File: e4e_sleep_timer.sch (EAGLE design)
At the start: 22 parts, among them P1 XT60, P2 10129378-906001BLF, P3 XT30PW-F, Q1 PJA3416AE_R1_00001, U1 NUCLEO-G071RB, U2 1224-5-150W

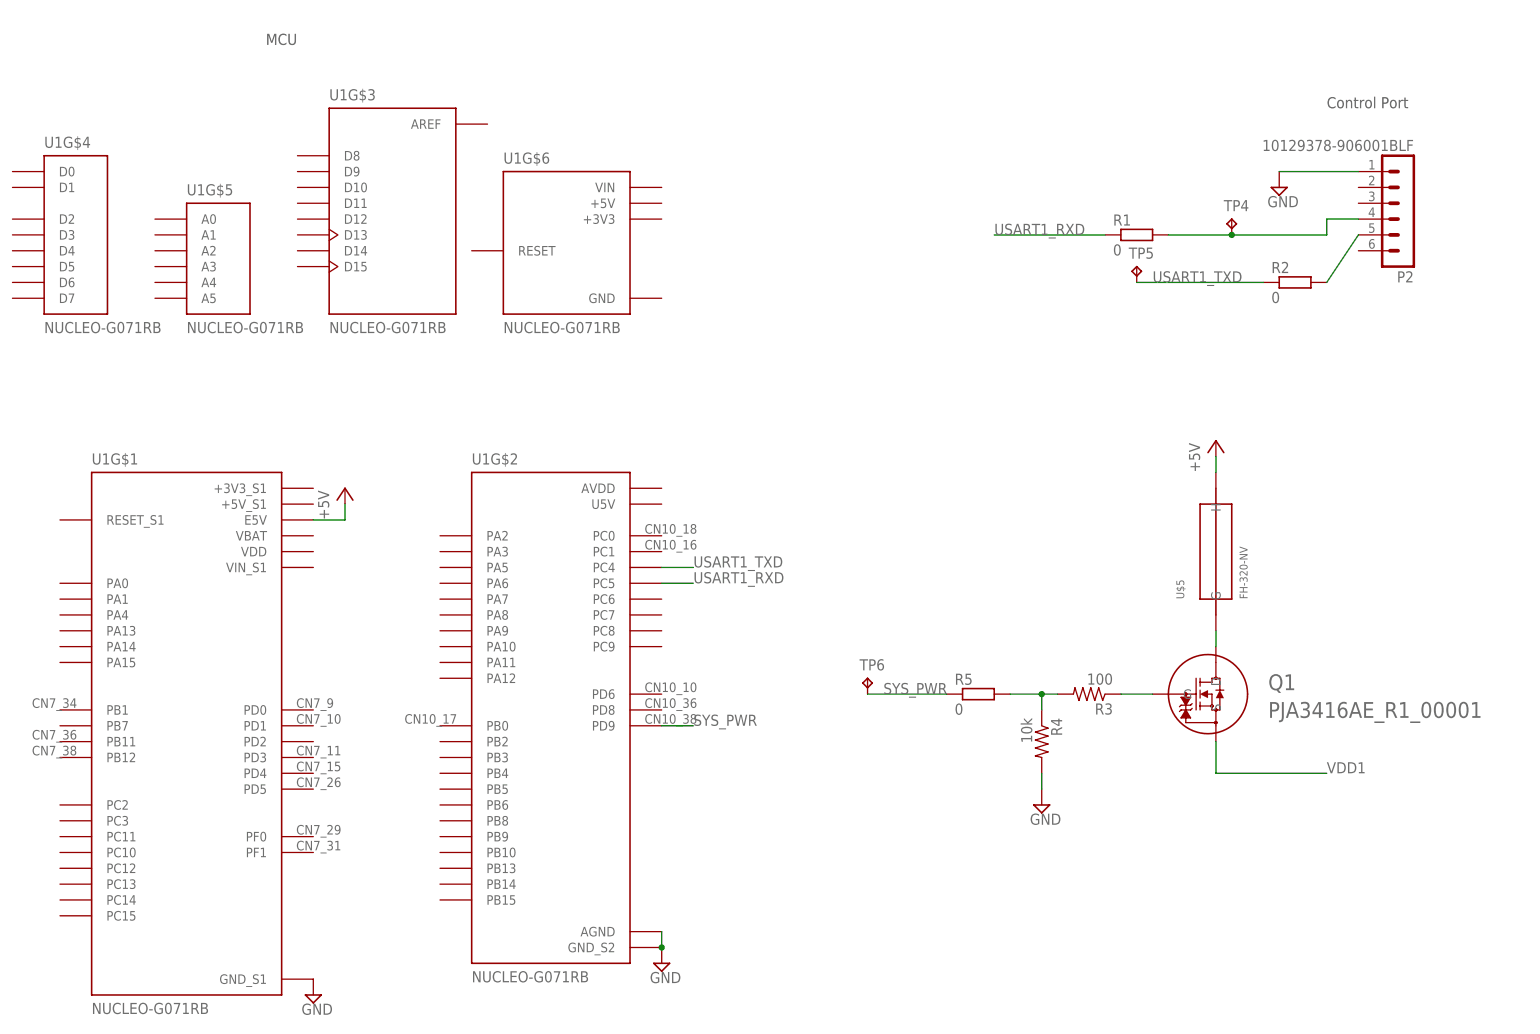
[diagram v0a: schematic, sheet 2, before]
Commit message: Finished PCB review
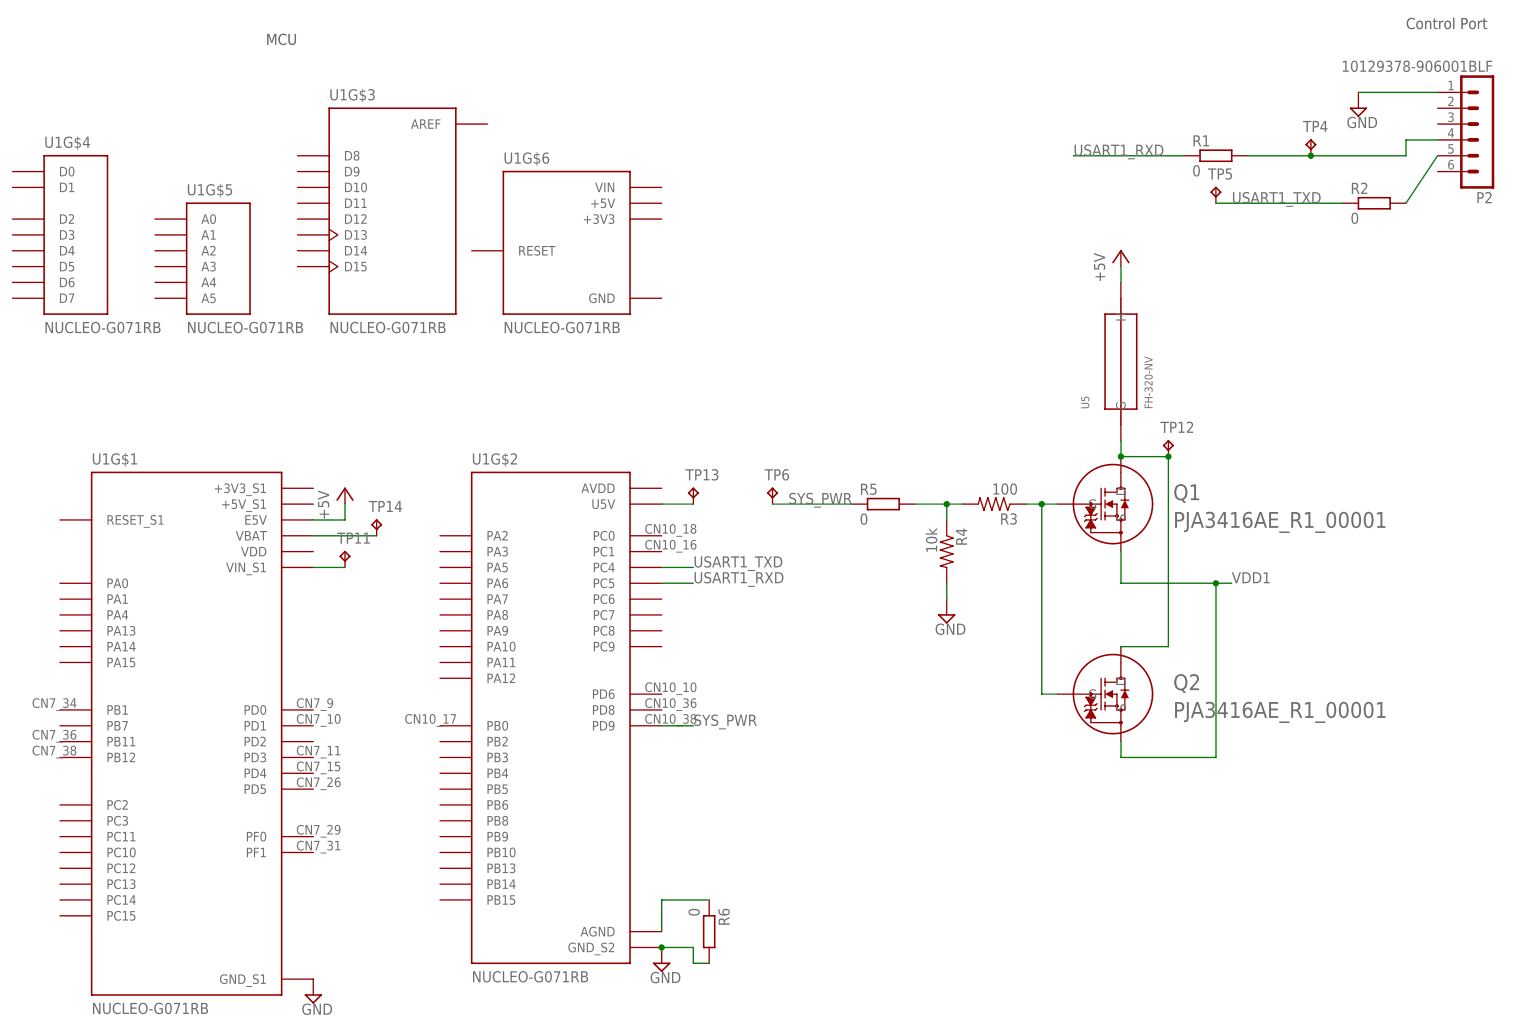
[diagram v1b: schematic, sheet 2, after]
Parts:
- removed U$5: FH-320-NV, fuses:FH-320-NV
- added Q2: PJA3416AE_R1_00001, PJA3416AE_R1_00001:PJA3416AE_R1_00001
- added R6: 0, rcl:R-EU_R0603
- added TP11, TP12, TP13, TP14: TPTP20R, testpad:TPTP20R
- added U5: FH-320-NV, fuses:FH-320-NV
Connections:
- new net N$6: TP11.TP, U1G$1.VIN_S1
- new net N$7: R6.1, U1G$2.AGND
- new net N$8: TP13.TP, U1G$2.U5V
- new net N$9: TP14.TP, U1G$1.VBAT
- net +5V: now also U5.H; no longer U$5.H
- net GND: now also R6.2; no longer U1G$2.AGND
- net N$2: now also Q2.G
- net N$5: now also Q2.D, TP12.TP, U5.G; no longer U$5.G
- net VDD1: now also Q2.S
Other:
- moved on the sheet: P2, Q1, R1, R2, R3, R4, R5, TP4, TP5, TP6
